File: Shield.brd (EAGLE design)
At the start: 99.1 x 68.6 mm, 71 parts

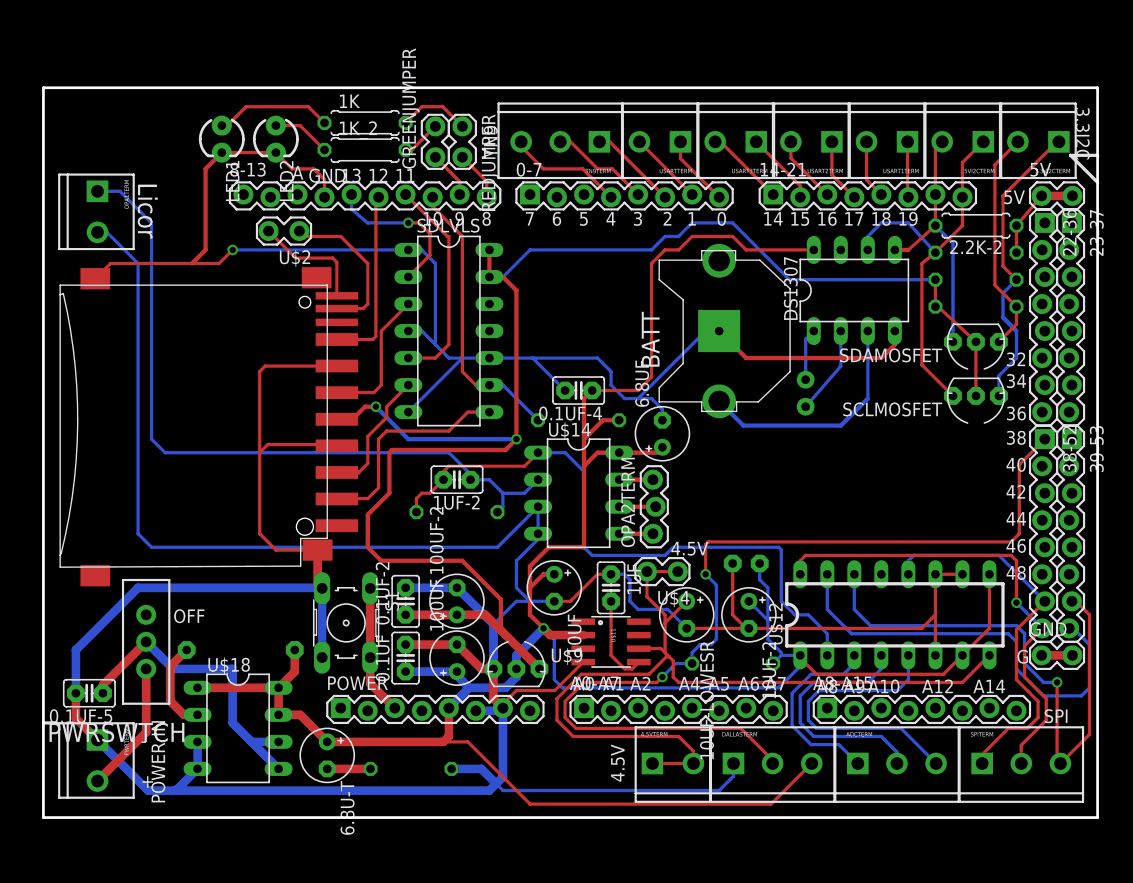
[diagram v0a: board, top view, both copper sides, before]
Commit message: Beginning Board Revision 2
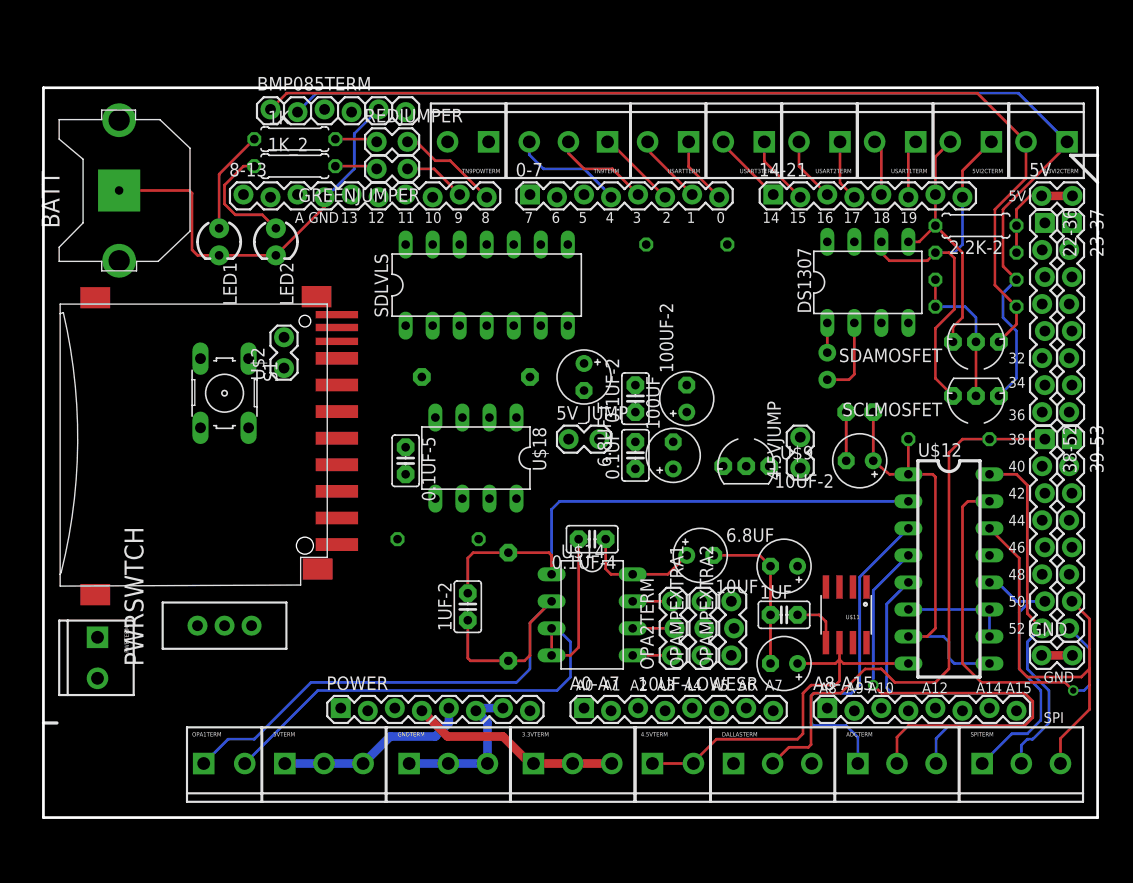
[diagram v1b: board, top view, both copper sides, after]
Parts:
- removed 6.8U-T: CES, LEMS:E2,5-5
- removed U$4: 2PHN, LEMS:2PH
- added 3.3VTERM, 5VTERM, GNDTERM: 3PHS, LEMS:SCREWTERMINAL-3.5MM-3_LOCK.007S
- added 4.5VJUMP, 5V_JUMP: 2PJN, LEMS:2PH
- added 6.8UF-T: CES, LEMS:E2,5-5
- added BMP085TERM: 6PHN, LEMS:6PH
- added OPAMPEXTRA1, OPAMPEXTRA2: 3PHN, LEMS:3PH
- added TN9POWTERM: 2PHS, LEMS:SCREWTERMINAL-3.5MM-2_LOCK
- 44.2K: value RESISTORT -> RESISTORN; device LEMS:0207/7 -> LEMS:0207/10
- moved BATT 57.9 mm to (7.11, 58.9)
- moved OPA1TERM 54.5 mm to (15.2, 5.08), turned to 0 degrees
- moved 0.1UF-5 36.9 mm to (34.0, 33.5), turned to 270 degrees
- moved 250K 33.9 mm to (40.6, 41.4)
- moved U$18 33.8 mm to (40.6, 33.8), turned to 180 degrees
- moved 4.7K 29.3 mm to (85.1, 35.6), turned to 0 degrees
- moved U$9 28.8 mm to (66.0, 33.0)
- moved 0.1UF 28.8 mm to (55.6, 34.0)
- moved 0.1UF-2 28.8 mm to (55.6, 39.4)
- moved 100UF-2 28.8 mm to (60.5, 39.4)
- moved 100UF 27.9 mm to (59.2, 34.0)
- moved S1 24.4 mm to (17.0, 39.9)
- moved U$11 22.2 mm to (75.4, 19.1), turned to 180 degrees
- moved 1 21.7 mm to (37.1, 26.2)
- moved 10UF 21.7 mm to (69.6, 23.6), turned to 180 degrees
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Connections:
- new net 5VOUT: 250K.2, 5V_JUMP.1, 6.8UF-T.+, U$18.1, U$18.7, U$18.8
- new net EOC: BMP085TERM.4
- new net XCLR: BMP085TERM.3
- net 3.3V: now also BMP085TERM.6
- net 3.3V_SCL: now also BMP085TERM.2
- net 3.3V_SDA: now also BMP085TERM.1
- net 4.5V: now also 4.5VJUMP.1; no longer U$4.1, U$4.2
- net 5V: now also 5VTERM.1, 5VTERM.2, 5VTERM.3, 5V_JUMP.2, TN9POWTERM.2; no longer 250K.2, 6.8U-T.+, U$18.1, U$18.7, U$18.8
- net AREF: now also 4.5VJUMP.2
- net GND: now also BMP085TERM.5, GNDTERM.1, GNDTERM.2, GNDTERM.3, TN9POWTERM.1
- net MEGA3.3V: now also 3.3VTERM.1, 3.3VTERM.2, 3.3VTERM.3
- net N$7: now also 6.8UF-T.-; no longer 6.8U-T.-
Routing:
- net GND: track 482.6 -> 138.3 mm, vias 1 -> 0
- net 5V: track 252.7 -> 80.5 mm, vias 1 -> 0
- net 3.3V: track 151.2 -> 14.1 mm, vias 2 -> 0
- net 3.3V_SCL: track 28.4 -> 103.6 mm
- net 3.3V_SDA: track 21.2 -> 95.1 mm
- net 4.5V: track 83.5 -> 37.5 mm
- net D38: track 89.3 -> 53.8 mm, vias 2 -> 0
- net N$8: track 29.4 -> 0.00 mm
- net SS_SOFT: track 26.5 -> 0.00 mm
- net CH2: track 23.8 -> 46.7 mm, vias 0 -> 1
- net VBAT: track 22.3 -> 0.00 mm
- net SD_CSIN: track 20.4 -> 0.00 mm
- net MOSI_SOFT: track 20.2 -> 0.00 mm
- net MEGA3.3V: track 0.00 -> 19.9 mm
- net MISO_SOFT: track 17.0 -> 0.00 mm
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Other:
- board text added: "50"
- board text added: "52"
- board text added: "A15"
- board text added: "A3"
- board text removed: "+"
- board text removed: "-"
- board text removed: "3.3I2C"
- board text removed: "4.5V"
- board text removed: "G"
- board text removed: "Licor"
- board text removed: "OFF"
- board text removed: "POWER IN"
- board text removed: "TN9"
